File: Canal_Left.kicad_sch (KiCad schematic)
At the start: 0 parts

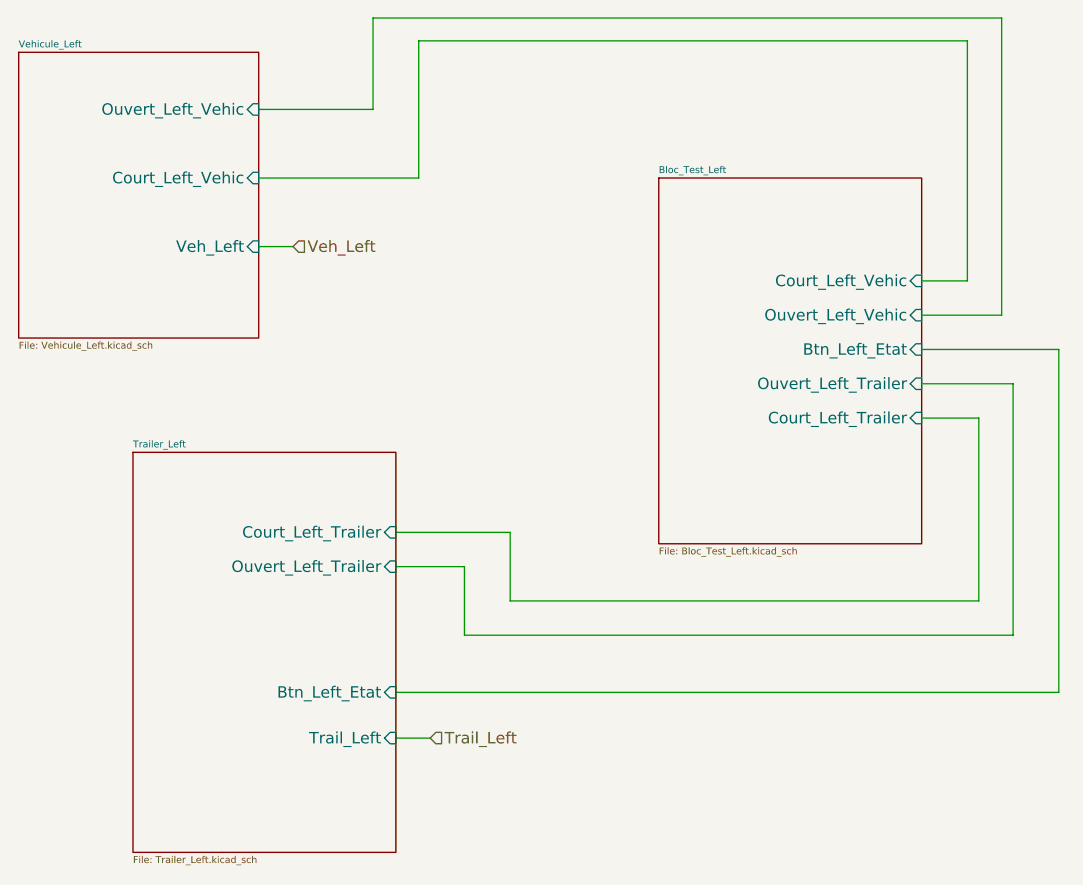
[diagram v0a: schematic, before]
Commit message: Add files via upload
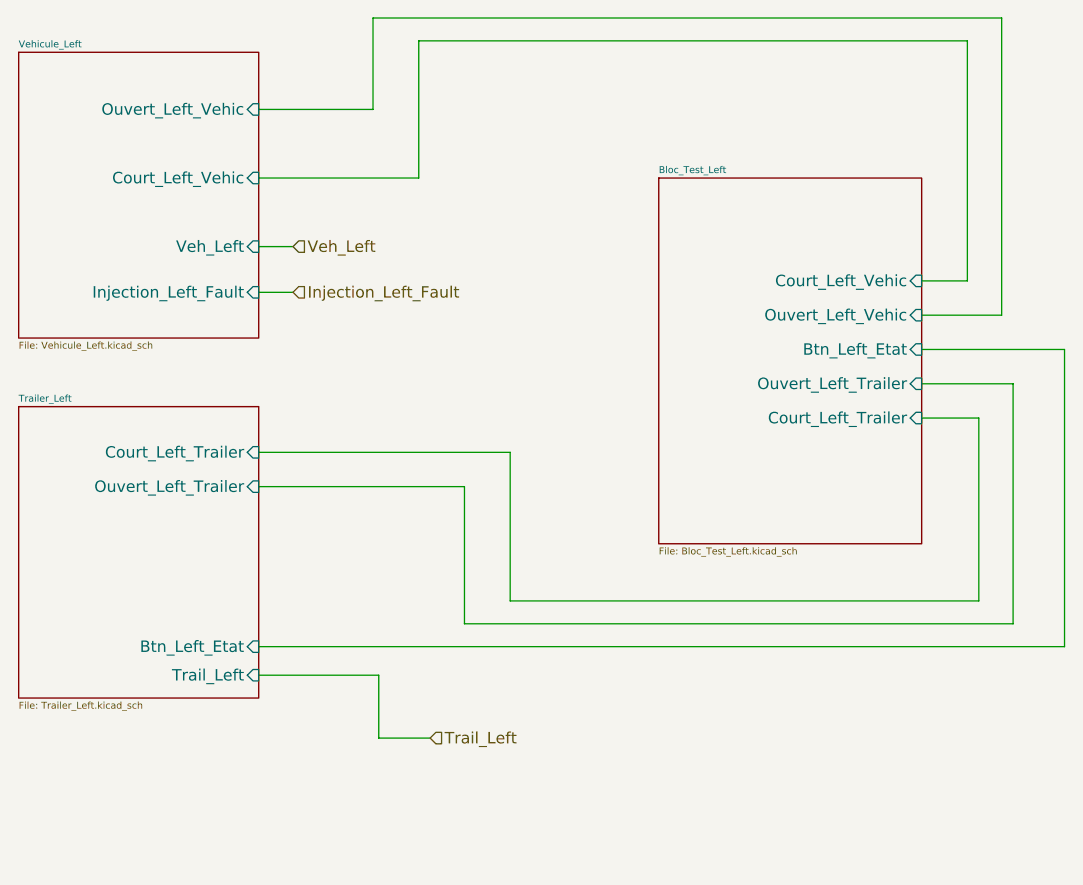
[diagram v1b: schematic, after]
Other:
- sheet Vehicule_Left ports: added Injection_Left_Fault; removed none
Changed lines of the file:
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@@
 	(wire
 		(pts
-			(xy 67.31 77.47) (xy 67.31 85.09)
-		)
-		(stroke
-			(width 0)
-			(type default)
-		)
-	)
-	(wire
-		(pts
-			(xy 59.69 96.52) (xy 63.5 96.52)
-		)
-		(stroke
-			(width 0)
-			(type default)
-		)
-	)
-	(wire
-		(pts
-			(xy 59.69 77.47) (xy 67.31 77.47)
+			(xy 67.31 68.58) (xy 67.31 83.82)
+		)
+		(stroke
+			(width 0)
+			(type default)
+		)
+	)
+	(wire
+		(pts
+			(xy 44.45 89.535) (xy 57.785 89.535)
+		)
+		(stroke
+			(width 0)
+			(type default)
+		)
+	)
+	(wire
+		(pts
+			(xy 44.45 68.58) (xy 67.31 68.58)
 		)
 		(stroke
@@
 	(wire
 		(pts
+			(xy 57.785 96.52) (xy 63.5 96.52)
+		)
+		(stroke
+			(width 0)
+			(type default)
+		)
+	)
+	(wire
+		(pts
 			(xy 44.45 34.29) (xy 62.23 34.29)
 		)
@@
 	(wire
 		(pts
-			(xy 72.39 73.66) (xy 72.39 81.28)
-		)
-		(stroke
-			(width 0)
-			(type default)
-		)
-	)
-	(wire
-		(pts
-			(xy 59.69 91.44) (xy 133.35 91.44)
-		)
-		(stroke
-			(width 0)
-			(type default)
-		)
-	)
-	(wire
-		(pts
-			(xy 133.35 53.34) (xy 133.35 91.44)
+			(xy 72.39 64.77) (xy 72.39 81.28)
+		)
+		(stroke
+			(width 0)
+			(type default)
+		)
+	)
+	(wire
+		(pts
+			(xy 44.45 86.36) (xy 133.985 86.36)
+		)
+		(stroke
+			(width 0)
+			(type default)
+		)
+	)
+	(wire
+		(pts
+			(xy 57.785 89.535) (xy 57.785 96.52)
+		)
+		(stroke
+			(width 0)
+			(type default)
+		)
+	)
+	(wire
+		(pts
+			(xy 133.985 53.34) (xy 133.985 86.36)
 		)
 		(stroke
@@
 	(wire
 		(pts
-			(xy 67.31 85.09) (xy 128.27 85.09)
+			(xy 67.31 83.82) (xy 128.27 83.82)
+		)
+		(stroke
+			(width 0)
+			(type default)
+		)
+	)
+	(wire
+		(pts
+			(xy 44.45 46.99) (xy 48.26 46.99)
 		)
 		(stroke
@@
 	(wire
 		(pts
-			(xy 59.69 73.66) (xy 72.39 73.66)
-		)
-		(stroke
-			(width 0)
-			(type default)
-		)
-	)
-	(wire
-		(pts
-			(xy 128.27 57.15) (xy 128.27 85.09)
+			(xy 44.45 64.77) (xy 72.39 64.77)
+		)
+		(stroke
+			(width 0)
+			(type default)
+		)
+	)
+	(wire
+		(pts
+			(xy 128.27 57.15) (xy 128.27 83.82)
 		)
 		(stroke
@@
 	(wire
 		(pts
-			(xy 118.11 53.34) (xy 133.35 53.34)
+			(xy 118.11 53.34) (xy 133.985 53.34)
 		)
 		(stroke
@@
 		)
 	)
+	(hierarchical_label "Injection_Left_Fault"
+		(shape input)
+		(at 48.26 46.99 0)
+		(effects
+			(font
+				(size 1.27 1.27)
+			)
+			(justify left)
+		)
+	)
 	(hierarchical_label "Veh_Left"
 		(shape input)
@@
 	)
 	(sheet
-		(at 30.48 64.77)
-		(size 29.21 44.45)
+		(at 17.78 59.69)
+		(size 26.67 32.385)
 		(exclude_from_sim no)
 		(in_bom yes)
@@
 		)
 		(property "Sheetname" "Trailer_Left"
-			(at 30.48 64.3124 0)
+			(at 17.78 59.2324 0)
 			(show_name no)
 			(do_not_autoplace no)
@@
 		)
 		(property "Sheetfile" "Trailer_Left.kicad_sch"
-			(at 30.48 109.6014 0)
+			(at 17.78 92.4564 0)
 			(show_name no)
 			(do_not_autoplace no)
@@
 		)
 		(pin "Trail_Left" input
-			(at 59.69 96.52 0)
+			(at 44.45 89.535 0)
 			(effects
 				(font
@@
 		)
 		(pin "Btn_Left_Etat" input
-			(at 59.69 91.44 0)
+			(at 44.45 86.36 0)
 			(effects
 				(font
@@
 		)
 		(pin "Ouvert_Left_Trailer" input
-			(at 59.69 77.47 0)
+			(at 44.45 68.58 0)
 			(effects
 				(font
@@
 		)
 		(pin "Court_Left_Trailer" input
-			(at 59.69 73.66 0)
+			(at 44.45 64.77 0)
 			(effects
 				(font
@@
 			(effects
 				(font
+					(size 1.27 1.27)
+				)
+				(justify right)
+			)
+		)
+		(pin "Injection_Left_Fault" input
+			(at 44.45 46.99 0)
+			(effects
+				(font

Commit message: Add files via upload
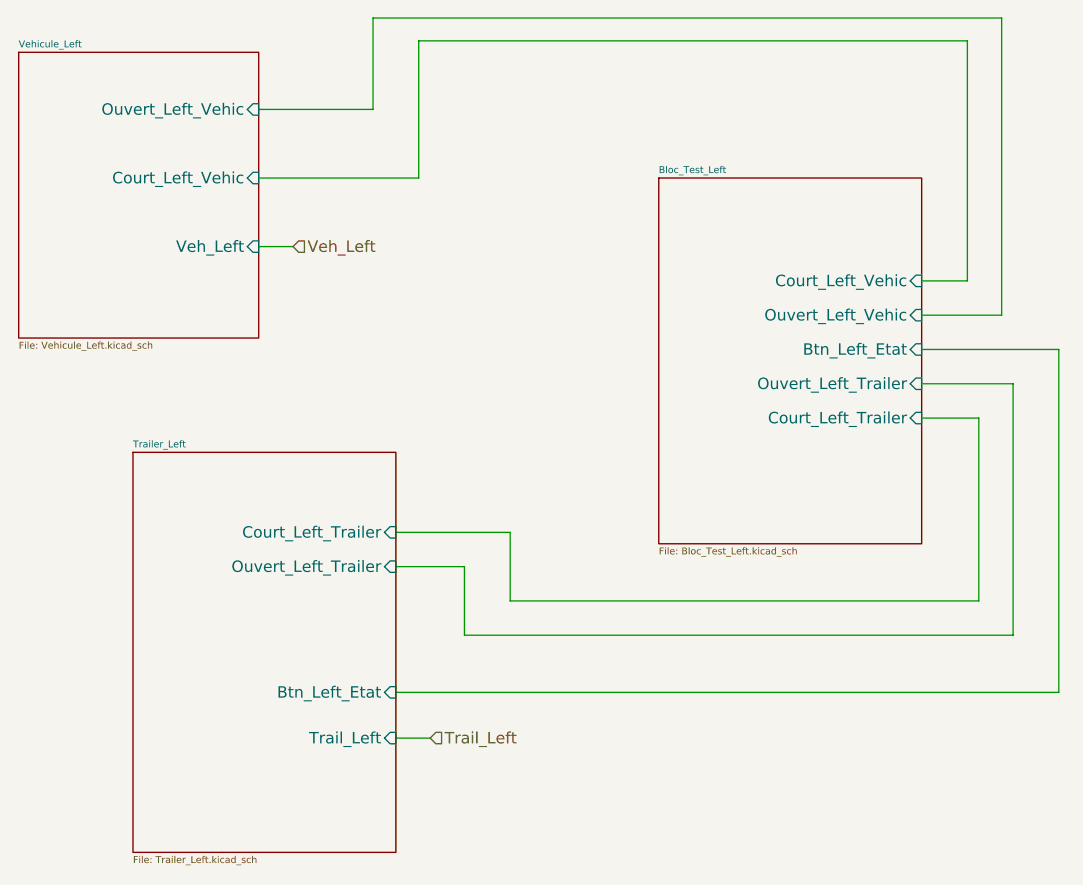
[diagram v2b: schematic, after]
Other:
- sheet Vehicule_Left ports: added none; removed Injection_Left_Fault
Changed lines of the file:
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@@
 	(wire
 		(pts
-			(xy 67.31 68.58) (xy 67.31 83.82)
-		)
-		(stroke
-			(width 0)
-			(type default)
-		)
-	)
-	(wire
-		(pts
-			(xy 44.45 89.535) (xy 57.785 89.535)
-		)
-		(stroke
-			(width 0)
-			(type default)
-		)
-	)
-	(wire
-		(pts
-			(xy 44.45 68.58) (xy 67.31 68.58)
+			(xy 67.31 77.47) (xy 67.31 85.09)
+		)
+		(stroke
+			(width 0)
+			(type default)
+		)
+	)
+	(wire
+		(pts
+			(xy 59.69 96.52) (xy 63.5 96.52)
+		)
+		(stroke
+			(width 0)
+			(type default)
+		)
+	)
+	(wire
+		(pts
+			(xy 59.69 77.47) (xy 67.31 77.47)
 		)
 		(stroke
@@
 	(wire
 		(pts
-			(xy 57.785 96.52) (xy 63.5 96.52)
-		)
-		(stroke
-			(width 0)
-			(type default)
-		)
-	)
-	(wire
-		(pts
 			(xy 44.45 34.29) (xy 62.23 34.29)
 		)
@@
 	(wire
 		(pts
-			(xy 72.39 64.77) (xy 72.39 81.28)
-		)
-		(stroke
-			(width 0)
-			(type default)
-		)
-	)
-	(wire
-		(pts
-			(xy 44.45 86.36) (xy 133.985 86.36)
-		)
-		(stroke
-			(width 0)
-			(type default)
-		)
-	)
-	(wire
-		(pts
-			(xy 57.785 89.535) (xy 57.785 96.52)
-		)
-		(stroke
-			(width 0)
-			(type default)
-		)
-	)
-	(wire
-		(pts
-			(xy 133.985 53.34) (xy 133.985 86.36)
+			(xy 72.39 73.66) (xy 72.39 81.28)
+		)
+		(stroke
+			(width 0)
+			(type default)
+		)
+	)
+	(wire
+		(pts
+			(xy 59.69 91.44) (xy 133.35 91.44)
+		)
+		(stroke
+			(width 0)
+			(type default)
+		)
+	)
+	(wire
+		(pts
+			(xy 133.35 53.34) (xy 133.35 91.44)
 		)
 		(stroke
@@
 	(wire
 		(pts
-			(xy 67.31 83.82) (xy 128.27 83.82)
-		)
-		(stroke
-			(width 0)
-			(type default)
-		)
-	)
-	(wire
-		(pts
-			(xy 44.45 46.99) (xy 48.26 46.99)
+			(xy 67.31 85.09) (xy 128.27 85.09)
 		)
 		(stroke
@@
 	(wire
 		(pts
-			(xy 44.45 64.77) (xy 72.39 64.77)
-		)
-		(stroke
-			(width 0)
-			(type default)
-		)
-	)
-	(wire
-		(pts
-			(xy 128.27 57.15) (xy 128.27 83.82)
+			(xy 59.69 73.66) (xy 72.39 73.66)
+		)
+		(stroke
+			(width 0)
+			(type default)
+		)
+	)
+	(wire
+		(pts
+			(xy 128.27 57.15) (xy 128.27 85.09)
 		)
 		(stroke
@@
 	(wire
 		(pts
-			(xy 118.11 53.34) (xy 133.985 53.34)
+			(xy 118.11 53.34) (xy 133.35 53.34)
 		)
 		(stroke
@@
 		)
 	)
-	(hierarchical_label "Injection_Left_Fault"
-		(shape input)
-		(at 48.26 46.99 0)
-		(effects
-			(font
-				(size 1.27 1.27)
-			)
-			(justify left)
-		)
-	)
 	(hierarchical_label "Veh_Left"
 		(shape input)
@@
 	)
 	(sheet
-		(at 17.78 59.69)
-		(size 26.67 32.385)
+		(at 30.48 64.77)
+		(size 29.21 44.45)
 		(exclude_from_sim no)
 		(in_bom yes)
@@
 		)
 		(property "Sheetname" "Trailer_Left"
-			(at 17.78 59.2324 0)
+			(at 30.48 64.3124 0)
 			(show_name no)
 			(do_not_autoplace no)
@@
 		)
 		(property "Sheetfile" "Trailer_Left.kicad_sch"
-			(at 17.78 92.4564 0)
+			(at 30.48 109.6014 0)
 			(show_name no)
 			(do_not_autoplace no)
@@
 		)
 		(pin "Trail_Left" input
-			(at 44.45 89.535 0)
+			(at 59.69 96.52 0)
 			(effects
 				(font
@@
 		)
 		(pin "Btn_Left_Etat" input
-			(at 44.45 86.36 0)
+			(at 59.69 91.44 0)
 			(effects
 				(font
@@
 		)
 		(pin "Ouvert_Left_Trailer" input
-			(at 44.45 68.58 0)
+			(at 59.69 77.47 0)
 			(effects
 				(font
@@
 		)
 		(pin "Court_Left_Trailer" input
-			(at 44.45 64.77 0)
+			(at 59.69 73.66 0)
 			(effects
 				(font
@@
 			(effects
 				(font
-					(size 1.27 1.27)
-				)
-				(justify right)
-			)
-		)
-		(pin "Injection_Left_Fault" input
-			(at 44.45 46.99 0)
-			(effects
-				(font

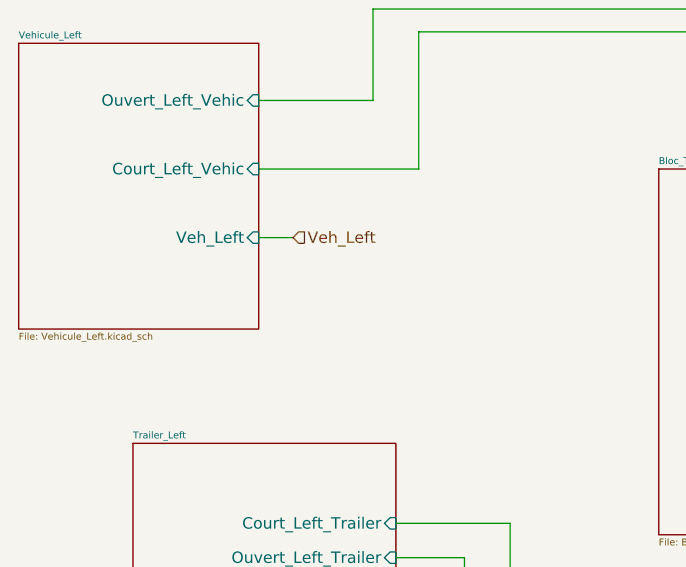
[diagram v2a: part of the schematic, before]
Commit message: Add files via upload
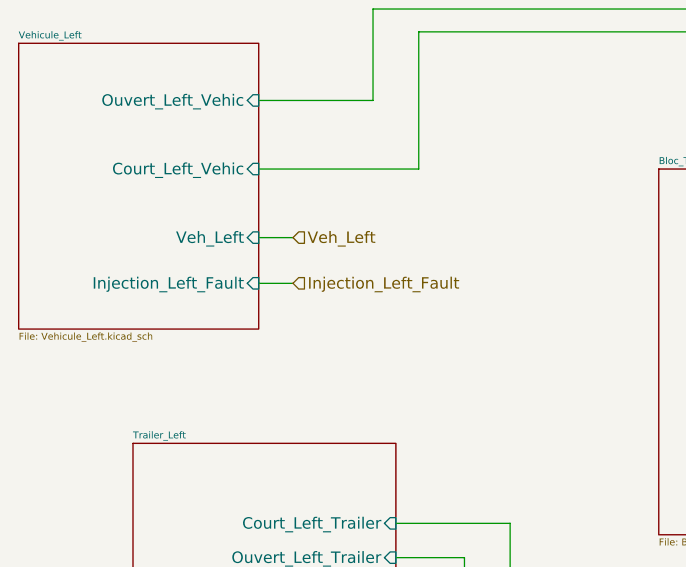
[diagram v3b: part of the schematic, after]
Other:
- sheet Vehicule_Left ports: added Injection_Left_Fault; removed none
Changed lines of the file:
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@@
+	(wire
+		(pts
+			(xy 44.45 46.99) (xy 48.26 46.99)
+		)
+		(stroke
+			(width 0)
+			(type default)
+		)
+	)
 	(wire
 		(pts
@@
 		(shape input)
 		(at 63.5 96.52 0)
+		(effects
+			(font
+				(size 1.27 1.27)
+			)
+			(justify left)
+		)
+	)
+	(hierarchical_label "Injection_Left_Fault"
+		(shape input)
+		(at 48.26 46.99 0)
 		(effects
 			(font
@@
 			(effects
 				(font
+					(size 1.27 1.27)
+				)
+				(justify right)
+			)
+		)
+		(pin "Injection_Left_Fault" input
+			(at 44.45 46.99 0)
+			(effects
+				(font

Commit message: Add files via upload
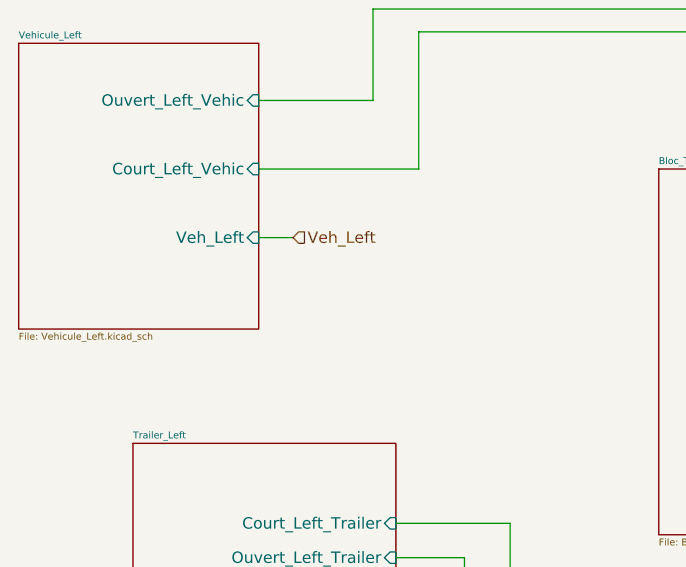
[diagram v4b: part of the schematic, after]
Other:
- sheet Vehicule_Left ports: added none; removed Injection_Left_Fault
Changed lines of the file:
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@@
-	(wire
-		(pts
-			(xy 44.45 46.99) (xy 48.26 46.99)
-		)
-		(stroke
-			(width 0)
-			(type default)
-		)
-	)
 	(wire
 		(pts
@@
 		(shape input)
 		(at 63.5 96.52 0)
-		(effects
-			(font
-				(size 1.27 1.27)
-			)
-			(justify left)
-		)
-	)
-	(hierarchical_label "Injection_Left_Fault"
-		(shape input)
-		(at 48.26 46.99 0)
 		(effects
 			(font
@@
 			(effects
 				(font
-					(size 1.27 1.27)
-				)
-				(justify right)
-			)
-		)
-		(pin "Injection_Left_Fault" input
-			(at 44.45 46.99 0)
-			(effects
-				(font
